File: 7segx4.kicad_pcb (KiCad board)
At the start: 2 copper layers, 203.2 x 86.4 mm, 5 parts, among them x1 HEADER2X7

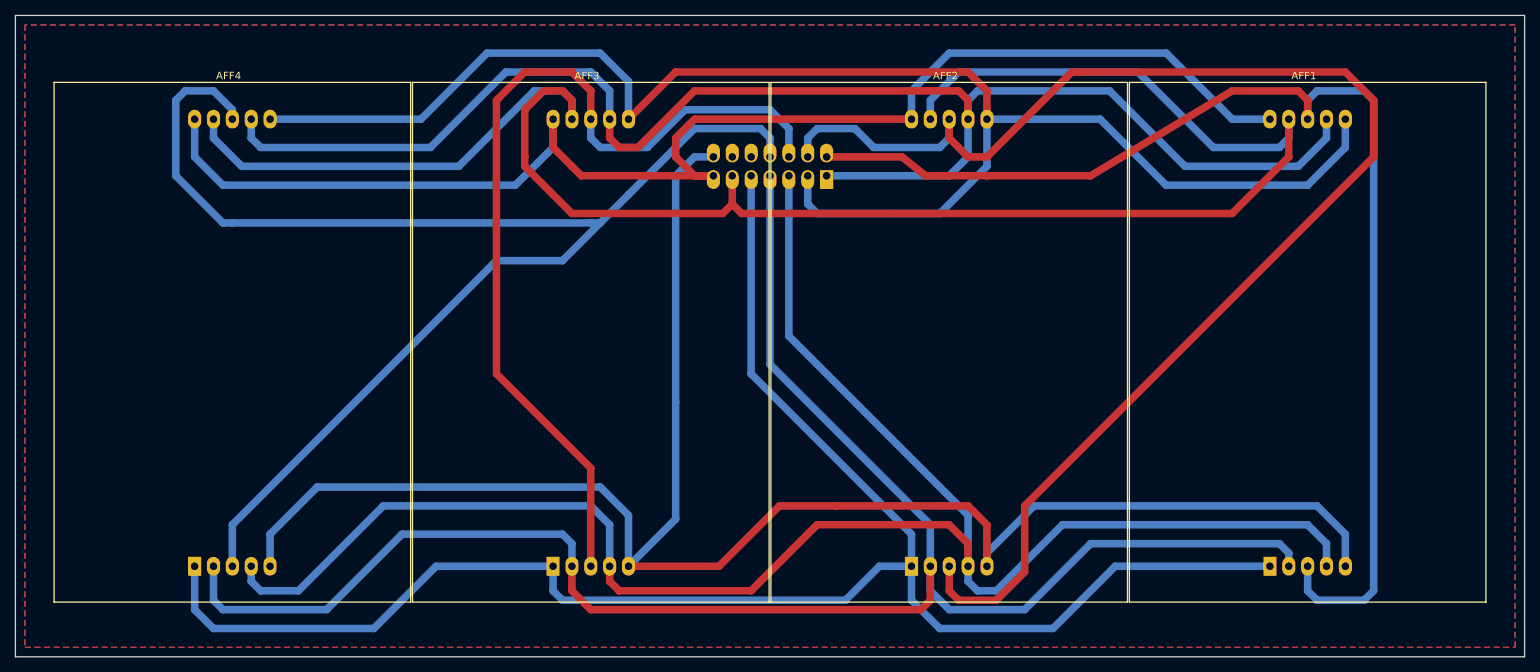
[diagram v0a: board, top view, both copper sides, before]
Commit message: track width+
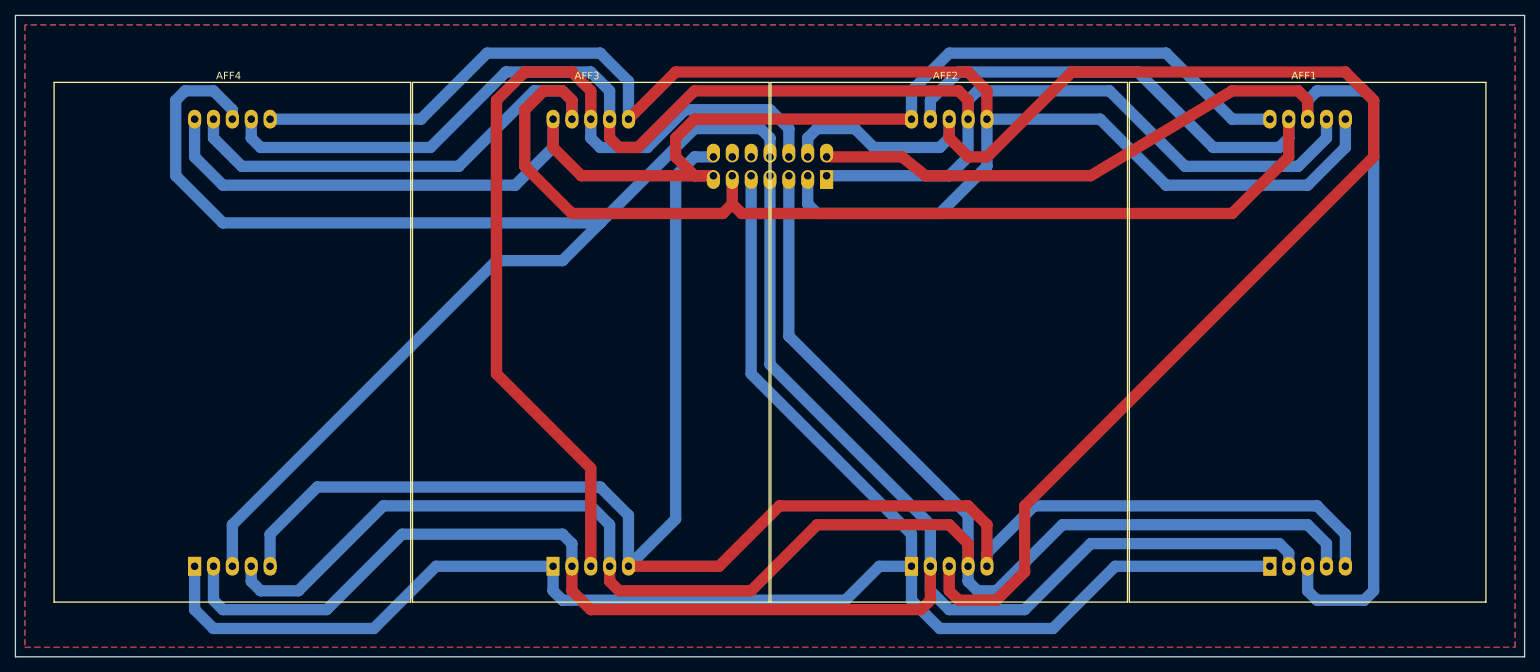
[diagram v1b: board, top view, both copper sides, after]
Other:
- net class Default: trace_width 1.016 -> 1.524
